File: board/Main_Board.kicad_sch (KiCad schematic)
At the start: 19 parts, among them J1 X Axis Encoder, J2 J2 Encoder, J3 J3 Encoder, J4 J4 Encoder, J5 Pitch Encoder, J6 I2C Bus, SW1 Enable Switch, U1 Teensy4.1_DEV-16771

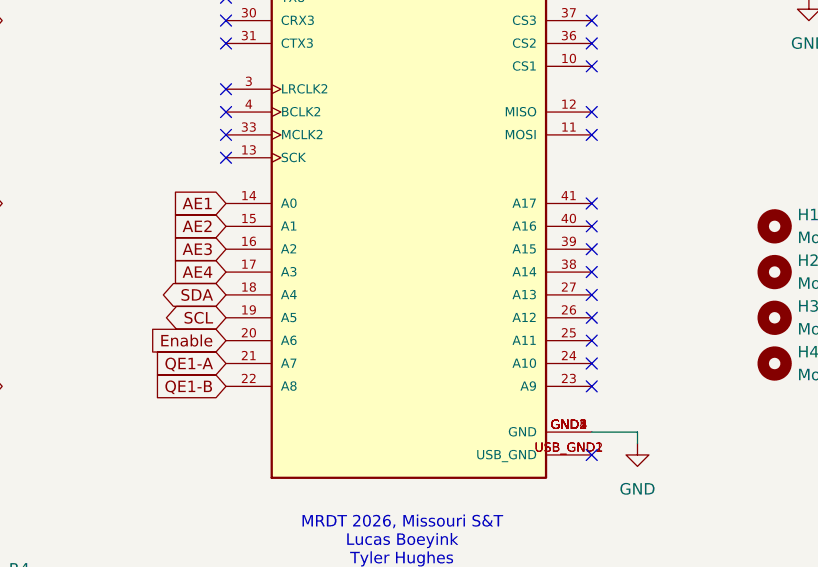
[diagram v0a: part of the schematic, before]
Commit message: Complete main board pre-review
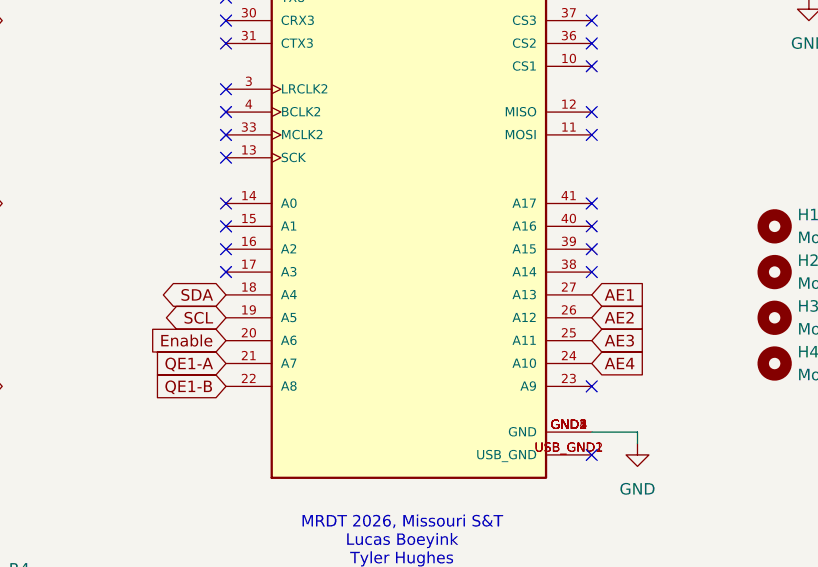
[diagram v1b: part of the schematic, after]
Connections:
- net AE1: now also U1.27 (A13); no longer U1.14 (A0)
- net AE2: now also U1.26 (A12); no longer U1.15 (A1)
- net AE3: now also U1.25 (A11); no longer U1.16 (A2)
- net AE4: now also U1.24 (A10); no longer U1.17 (A3)
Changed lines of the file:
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@@
-	)
-	(no_connect
-		(at 198.12 120.65)
 	)
 	(no_connect
@@
 	)
 	(no_connect
+		(at 157.48 115.57)
+	)
+	(no_connect
 		(at 157.48 105.41)
 	)
 	(no_connect
+		(at 157.48 113.03)
+	)
+	(no_connect
 		(at 157.48 72.39)
 	)
@@
 	)
 	(no_connect
-		(at 198.12 123.19)
-	)
-	(no_connect
 		(at 157.48 69.85)
 	)
@@
 	)
 	(no_connect
+		(at 157.48 118.11)
+	)
+	(no_connect
 		(at 198.12 46.99)
 	)
 	(no_connect
-		(at 198.12 125.73)
-	)
-	(no_connect
 		(at 157.48 102.87)
 	)
@@
 	)
 	(no_connect
-		(at 198.12 128.27)
+		(at 157.48 110.49)
 	)
 	(wire
@@
 	(global_label "AE2"
 		(shape input)
-		(at 157.48 113.03 180)
-		(fields_autoplaced yes)
-		(effects
-			(font
-				(size 1.27 1.27)
-			)
-			(justify right)
-		)
-		(property "Intersheetrefs" "${INTERSHEET_REFS}"
-			(at 151.0477 113.03 0)
-			(effects
-				(font
-					(size 1.27 1.27)
-				)
-				(justify right)
+		(at 198.12 123.19 0)
+		(fields_autoplaced yes)
+		(effects
+			(font
+				(size 1.27 1.27)
+			)
+			(justify left)
+		)
+		(property "Intersheetrefs" "${INTERSHEET_REFS}"
+			(at 204.5523 123.19 0)
+			(effects
+				(font
+					(size 1.27 1.27)
+				)
+				(justify left)
 				(hide yes)
 			)
@@
 	(global_label "AE4"
 		(shape input)
-		(at 157.48 118.11 180)
-		(fields_autoplaced yes)
-		(effects
-			(font
-				(size 1.27 1.27)
-			)
-			(justify right)
-		)
-		(property "Intersheetrefs" "${INTERSHEET_REFS}"
-			(at 151.0477 118.11 0)
-			(effects
-				(font
-					(size 1.27 1.27)
-				)
-				(justify right)
+		(at 198.12 128.27 0)
+		(fields_autoplaced yes)
+		(effects
+			(font
+				(size 1.27 1.27)
+			)
+			(justify left)
+		)
+		(property "Intersheetrefs" "${INTERSHEET_REFS}"
+			(at 204.5523 128.27 0)
+			(effects
+				(font
+					(size 1.27 1.27)
+				)
+				(justify left)
 				(hide yes)
 			)
@@
 	(global_label "AE1"
 		(shape input)
-		(at 157.48 110.49 180)
-		(fields_autoplaced yes)
-		(effects
-			(font
-				(size 1.27 1.27)
-			)
-			(justify right)
-		)
-		(property "Intersheetrefs" "${INTERSHEET_REFS}"
-			(at 151.0477 110.49 0)
-			(effects
-				(font
-					(size 1.27 1.27)
-				)
-				(justify right)
+		(at 198.12 120.65 0)
+		(fields_autoplaced yes)
+		(effects
+			(font
+				(size 1.27 1.27)
+			)
+			(justify left)
+		)
+		(property "Intersheetrefs" "${INTERSHEET_REFS}"
+			(at 204.5523 120.65 0)
+			(effects
+				(font
+					(size 1.27 1.27)
+				)
+				(justify left)
 				(hide yes)
 			)
@@
 	(global_label "AE3"
 		(shape input)
-		(at 157.48 115.57 180)
-		(fields_autoplaced yes)
-		(effects
-			(font
-				(size 1.27 1.27)
-			)
-			(justify right)
-		)
-		(property "Intersheetrefs" "${INTERSHEET_REFS}"
-			(at 151.0477 115.57 0)
-			(effects
-				(font
-					(size 1.27 1.27)
-				)
-				(justify right)
-				(hide yes)
-			)
+		(at 198.12 125.73 0)
+		(fields_autoplaced yes)
+		(effects
+			(font
+				(size 1.27 1.27)
+			)
+			(justify left)
+		)
+		(property "Intersheetrefs" "${INTERSHEET_REFS}"
+			(at 204.5523 125.73 0)
+			(effects
+				(font
+					(size 1.27 1.27)
+				)
+				(justify left)
+				(hide yes)
+			)
